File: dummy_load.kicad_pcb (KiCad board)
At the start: 2 copper layers, 16 parts, among them Q1 IRFZ44N

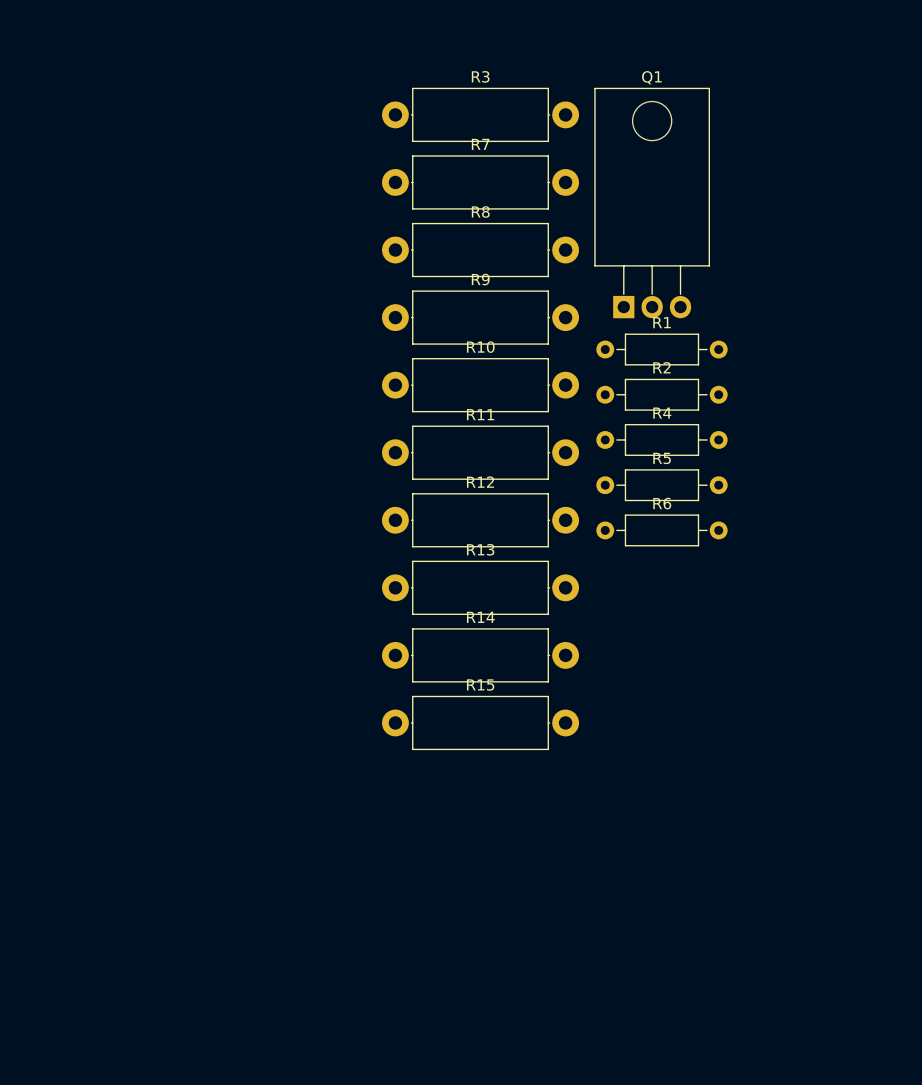
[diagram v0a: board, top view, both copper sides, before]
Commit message: Completada la version 1
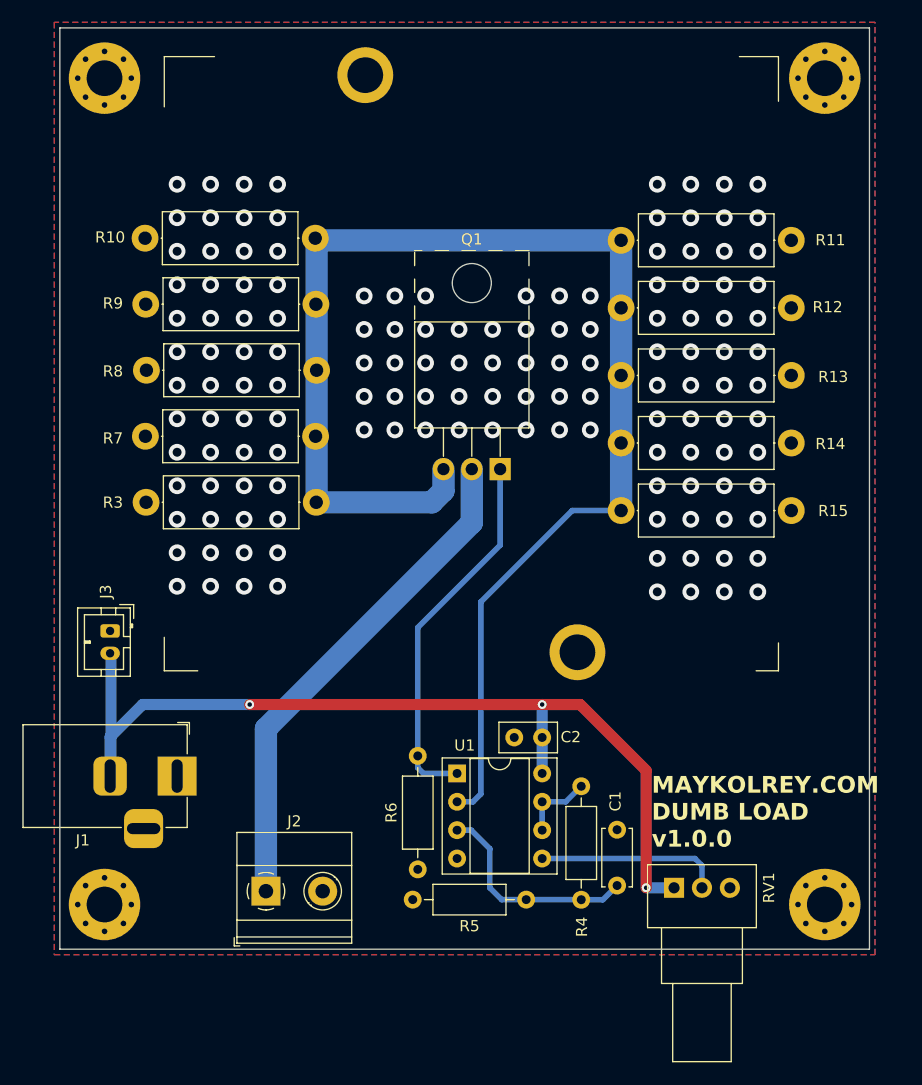
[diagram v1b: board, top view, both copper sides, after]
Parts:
- removed R1: 10k, Resistor_THT:R_Axial_DIN0207_L6.3mm_D2.5mm_P10.16mm_Horizontal
- removed R2: 2k, Resistor_THT:R_Axial_DIN0207_L6.3mm_D2.5mm_P10.16mm_Horizontal
- added C1: 1u, Capacitor_THT:C_Disc_D5.0mm_W2.5mm_P5.00mm, F.Cu at (156.9, 133.3)
- added C2: 100nF, Capacitor_THT:C_Disc_D5.0mm_W2.5mm_P2.50mm, F.Cu at (150.2, 120.0)
- added G***: LOGO, MR-footprint:logo_mr_6x6mm, F.Cu at (168.0, 119.2)
- added H1: MountingHole, MountingHole:MountingHole_3.2mm_M3_Pad_Via, F.Cu at (175.5, 61.0)
- added H2: MountingHole, MountingHole:MountingHole_3.2mm_M3_Pad_Via, F.Cu at (111.0, 61.0)
- added H3: MountingHole, MountingHole:MountingHole_3.2mm_M3_Pad_Via, F.Cu at (111.0, 135.0)
- added H4: MountingHole, MountingHole:MountingHole_3.2mm_M3_Pad_Via, F.Cu at (175.5, 135.0)
- added HS1: Heatsink, MR-footprint:disipador_VGA, F.Cu at (143.8, 86.6)
- added J1: Conn_01x02, Connector_BarrelJack:BarrelJack_Horizontal, F.Cu at (117.5, 123.5)
- added J2: Conn_01x02, TerminalBlock_Phoenix:TerminalBlock_Phoenix_MKDS-1,5-2-5.08_1x02_P5.08mm_Horizontal, F.Cu at (125.5, 133.8)
- added J3: PH_B2B-PH-K, Connector_JST:JST_PH_B2B-PH-K_1x02_P2.00mm_Vertical, F.Cu at (111.5, 110.5)
- added RV1: 5k, Potentiometer_THT:Potentiometer_Alps_RK09Y11_Single_Horizontal, F.Cu at (162.0, 133.5)
- added U1: LM358, Package_DIP:DIP-8_W7.62mm_Socket, F.Cu at (142.6, 123.3)
- Q1: footprint Package_TO_SOT_THT:TO-220-3_Horizontal_TabDown -> Package_TO_SOT_THT:TO-220-3_Horizontal_TabUp
- moved R4 41.2 mm to (153.7, 134.6), turned to 90 degrees
- moved R5 37.8 mm to (148.8, 134.6), turned to 180 degrees
- moved R3 35.4 mm to (130.0, 99.0), turned to 180 degrees
- moved R6 34.7 mm to (139.1, 131.8), turned to 90 degrees
- moved R11 27.8 mm to (157.3, 75.5)
- moved R12 27.8 mm to (157.3, 81.6)
- moved R13 27.8 mm to (157.3, 87.6)
- moved R14 27.8 mm to (157.3, 93.7)
- moved R15 27.8 mm to (157.3, 99.7)
- moved R7 23.8 mm to (129.9, 93.1), turned to 180 degrees
- moved Q1 18.3 mm to (146.4, 96.0), turned to 180 degrees
- moved R10 15.0 mm to (129.9, 75.3), turned to 180 degrees
- moved R8 12.9 mm to (130.0, 87.2), turned to 180 degrees
- moved R9 7.22 mm to (129.9, 81.2), turned to 180 degrees
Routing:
- net /vsense: track 0.00 -> 124.7 mm
- net +12V: track 0.00 -> 85.4 mm, vias 0 -> 3
- net Net-(J2-Pin_1): track 0.00 -> 45.4 mm
- net /vo: track 0.00 -> 33.5 mm
- net /vref: track 0.00 -> 19.5 mm
- net /vin: track 0.00 -> 16.6 mm
- net Net-(U1B--): track 0.00 -> 6.62 mm
- net GND: vias 0 -> 142
- added copper zone on B.Cu, net GND
- added copper zone on F.Cu, net GND
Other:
- board outline added: 72.5 x 82.5 mm
- board text added: "MAYKOLREY.COM DUMB LOAD ${REVISION}"
